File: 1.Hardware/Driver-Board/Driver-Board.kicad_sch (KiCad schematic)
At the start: 75 parts, among them J1 Conn_01x04, J2 Conn_01x02, J3 Conn_01x02, J4 Conn_01x04, J5 Conn_01x02, J6 Conn_01x02, Q1 FDN352AP, SW1 SW_Push, U1 MP2456, U2 MCP1700-3302E_SOT23, U3 TJA1051T-3, U4 AS5600, U5 TB67H450FNG,EL, U6 TB67H450FNG,EL, U7 STM32F103C6Tx, Y1 12MHz

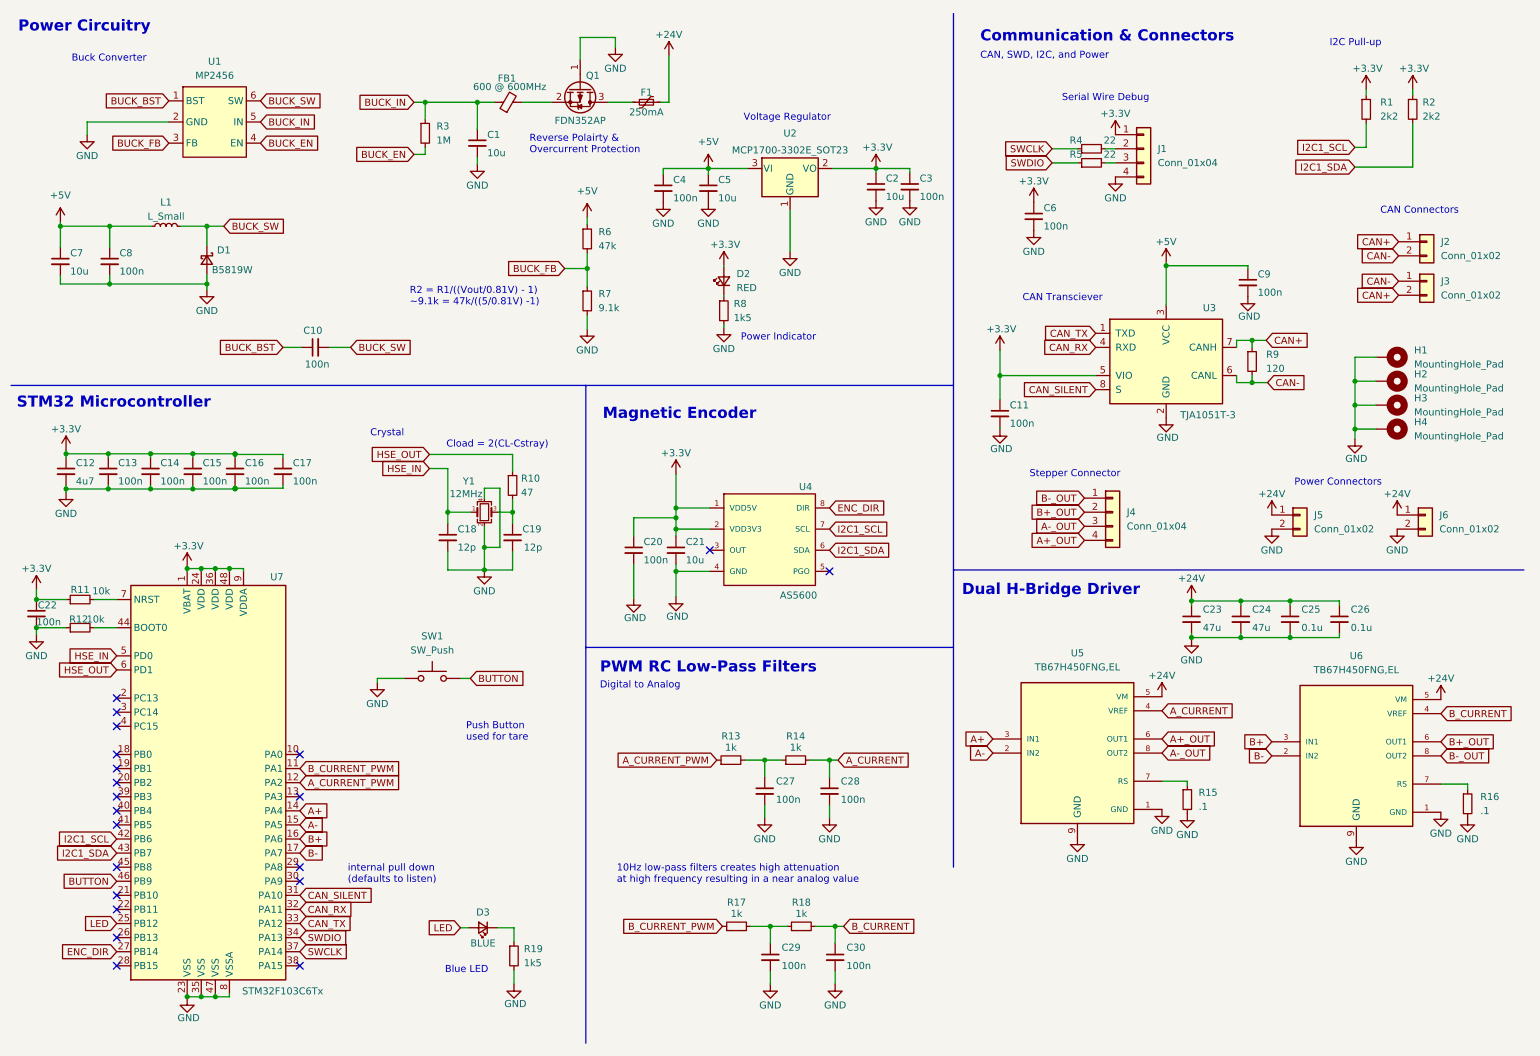
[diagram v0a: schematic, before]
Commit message: updated board
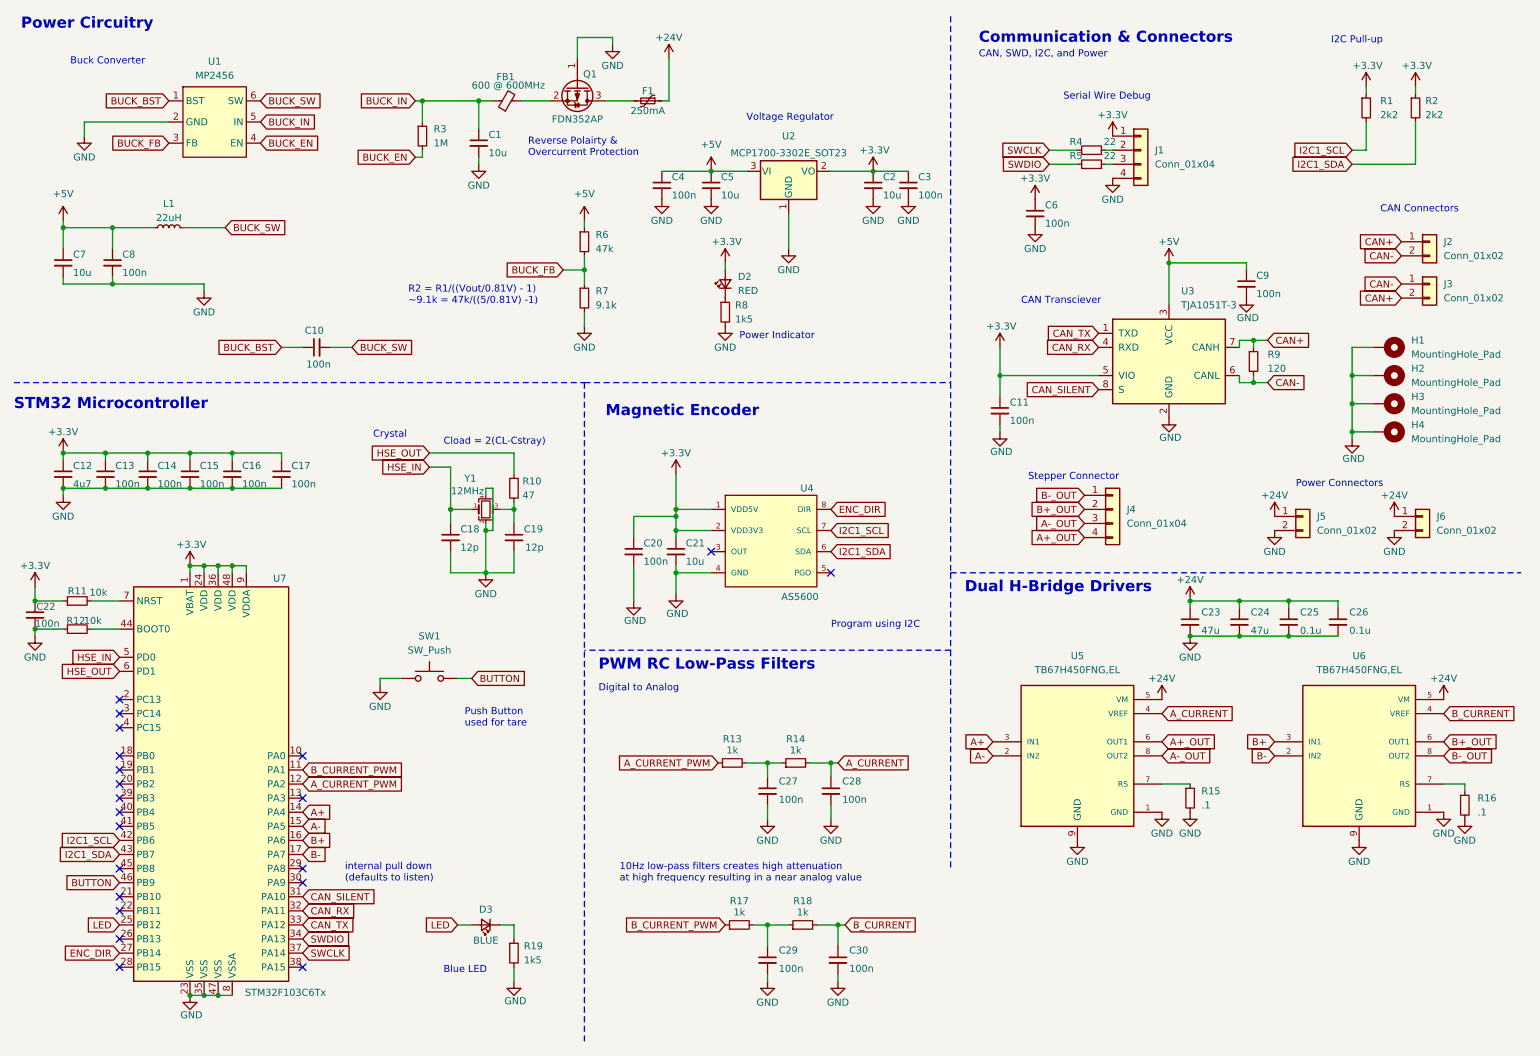
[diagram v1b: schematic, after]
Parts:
- removed D1: B5819W, Diode_SMD:D_SOD-123, symbol Device:D_Schottky_Small
- L1: value L_Small -> 22uH
- SW1: footprint Button_Switch_SMD:SW_SPST_TL3305B -> custom:KMR731NG LFS
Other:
- note added: "Dual H-Bridge Drivers"
- note added: "Program using I2C"
- note removed: "Dual H-Bridge Driver"
- moved on the sheet: C11, C12, C13, C14, C15, C16, C17, C18, C2, C23, C24, C25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
